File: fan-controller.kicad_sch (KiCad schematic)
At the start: 22 parts, among them J1 Conn_01x04_Pin, J2 Conn_01x04_Pin, J3 Conn_01x04_Pin, J4 12v, J5 Conn_01x04_Pin, Q1 Q_NMOS_GSD, Q2 Q_NMOS_GSD, Q3 Q_NMOS_GSD, U1 ESP32-S3-WROOM-1, U2 AMS1117-3.3

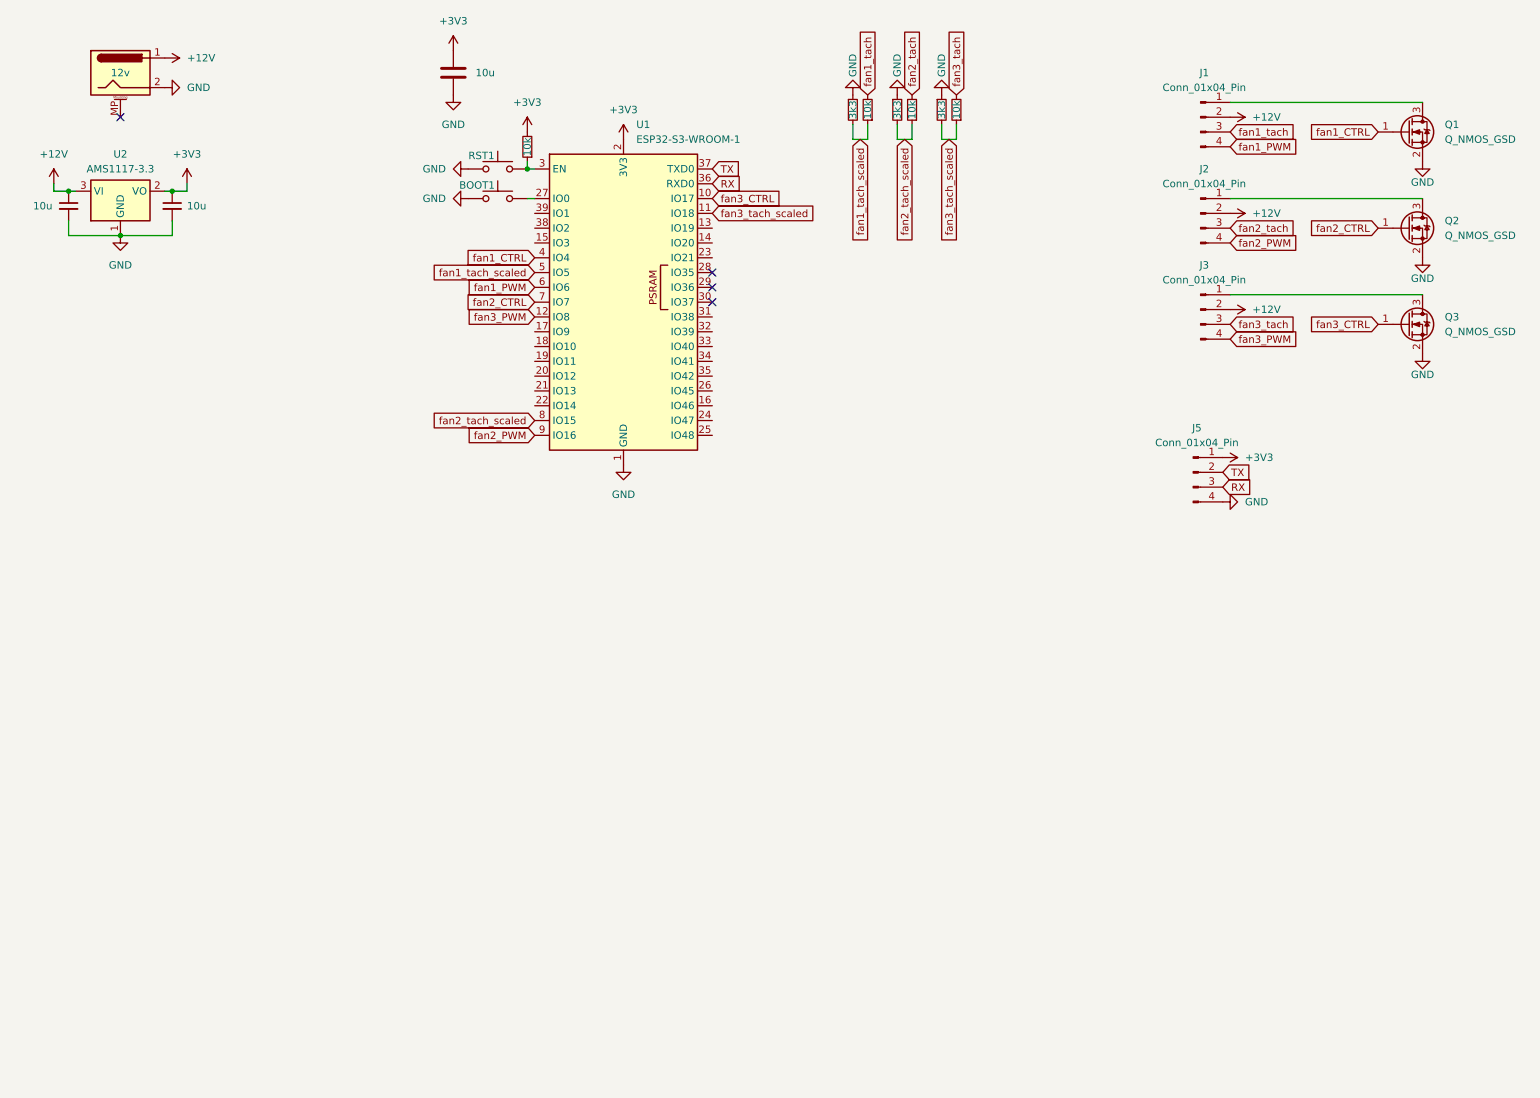
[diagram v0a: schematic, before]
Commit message: Add backup files, Final layout
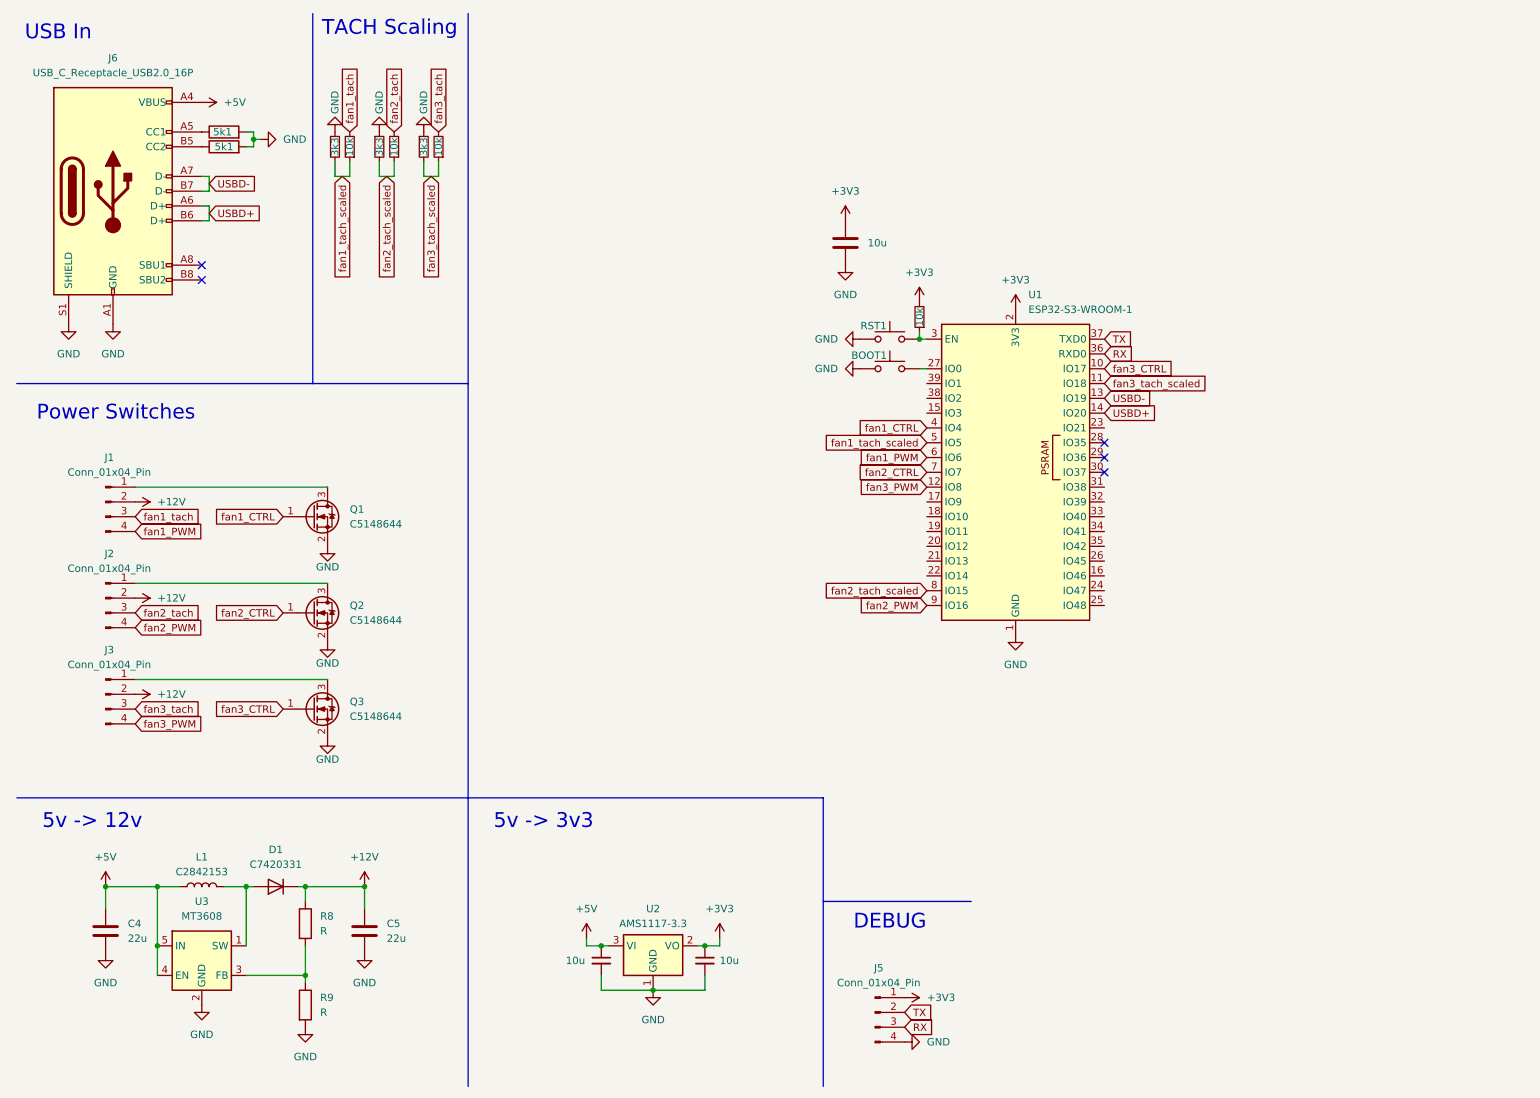
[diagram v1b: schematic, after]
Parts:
- removed J4: 12v, Connector_BarrelJack:BarrelJack_Horizontal, symbol Connector:Barrel_Jack_MountingPin
- added C4, C5: 22u, Capacitor_SMD:C_0805_2012Metric, symbol Device:C
- added D1: C7420331, Diode_SMD:D_SOD-323, symbol Device:D
- added J6: USB_C_Receptacle_USB2.0_16P, Connector_USB:USB_C_Receptacle_HRO_TYPE-C-31-M-12, symbol Connector:USB_C_Receptacle_USB2.0_16P
- added L1: C2842153, Inductor_SMD:L_Chilisin_BMRB00050518-B, symbol Device:L
- added R10, R11: 5k1, Resistor_SMD:R_0402_1005Metric, symbol Device:R
- added R8, R9: R, Resistor_SMD:R_0402_1005Metric, symbol Device:R
- added U3: MT3608, Package_TO_SOT_SMD:SOT-23-6, symbol Regulator_Switching:MT3608
- Q1, Q2, Q3: value Q_NMOS_GSD -> C5148644; footprint Package_TO_SOT_SMD:SOT-323_SC-70 -> Package_TO_SOT_SMD:SOT-523
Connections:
- net +12V: now also C5.1, D1.1 (K), R8.1; no longer C1.1, U2.3 (VI)
- net GND: now also C4.2, C5.2, J6.A1 (GND), J6.A12 (GND), J6.B1 (GND), J6.B12 (GND), J6.S1 (SHIELD), R10.2, R11.2, R9.2, U3.2 (GND)
- net USBD-: now reaches U1.13 (IO19)
- net USBD-: now also J6.A7 (D-), J6.B7 (D-)
- net USBD+: now reaches U1.14 (IO20)
- net USBD+: now also J6.A6 (D+), J6.B6 (D+)
- new net: D1.2 (A), L1.2, U3.1 (SW)
- new net: R8.2, R9.1, U3.3 (FB)
- new net: J6.A5 (CC1), R10.1
- new net: J6.B5 (CC2), R11.1
- new net +5V: C1.1, C4.1, J6.A4 (VBUS), J6.A9 (VBUS), J6.B4 (VBUS), J6.B9 (VBUS), L1.1, U2.3 (VI), U3.4 (EN), U3.5 (IN)
- no-connect marks 4 -> 5
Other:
- note added: "5v -> 12v"
- note added: "5v -> 3v3"
- note added: "DEBUG"
- note added: "Power Switches"
- note added: "TACH Scaling"
- note added: "USB In"
- moved on the sheet: BOOT1, J1, J2, J3, J5, Q1, Q2, Q3, RST1, U1, U2
